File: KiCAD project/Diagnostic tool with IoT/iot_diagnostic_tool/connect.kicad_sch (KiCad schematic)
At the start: 0 parts

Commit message: Update 03/03/23 - new schematic done
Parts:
- added J5: Debug, symbol Connector_Generic:Conn_02x05_Odd_Even
- added J7: OBD, symbol Connector:Conn_01x08_Socket
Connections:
- new net +12V: J7.8 (Pin_8)
- new net +3V3: J5.1 (Pin_1)
- new net CAN_H: J7.3 (Pin_3)
- new net CAN_L: J7.4 (Pin_4)
- new net DBG_RX: J5.5 (Pin_5)
- new net DBG_TX: J5.3 (Pin_3)
- new net GND: J5.10 (Pin_10), J5.7 (Pin_7), J5.9 (Pin_9), J7.2 (Pin_2), J7.5 (Pin_5)
- new net ISO_K: J7.6 (Pin_6)
- new net ISO_L: J7.7 (Pin_7)
- new net NRST: J5.8 (Pin_8)
- new net SWCLK: J5.4 (Pin_4)
- new net SWDIO: J5.2 (Pin_2)
- new net SWO: J5.6 (Pin_6)
- no-connect marks 0 -> 1
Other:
- note added: "Connectors"
- note added: "Debug"
- note added: "OBD"

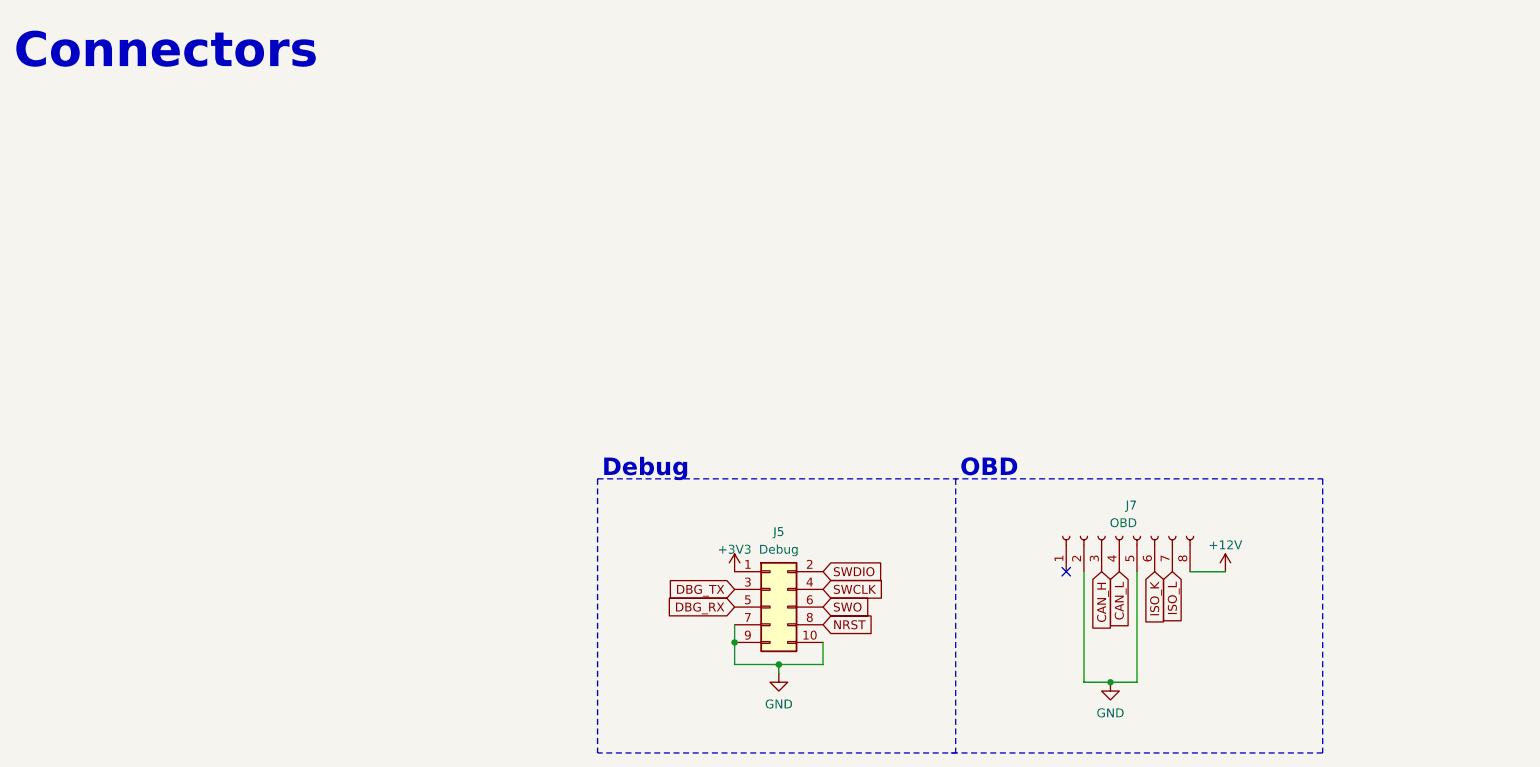
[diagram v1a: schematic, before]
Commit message: Update 06/03/23 - new board layout WIP 70%
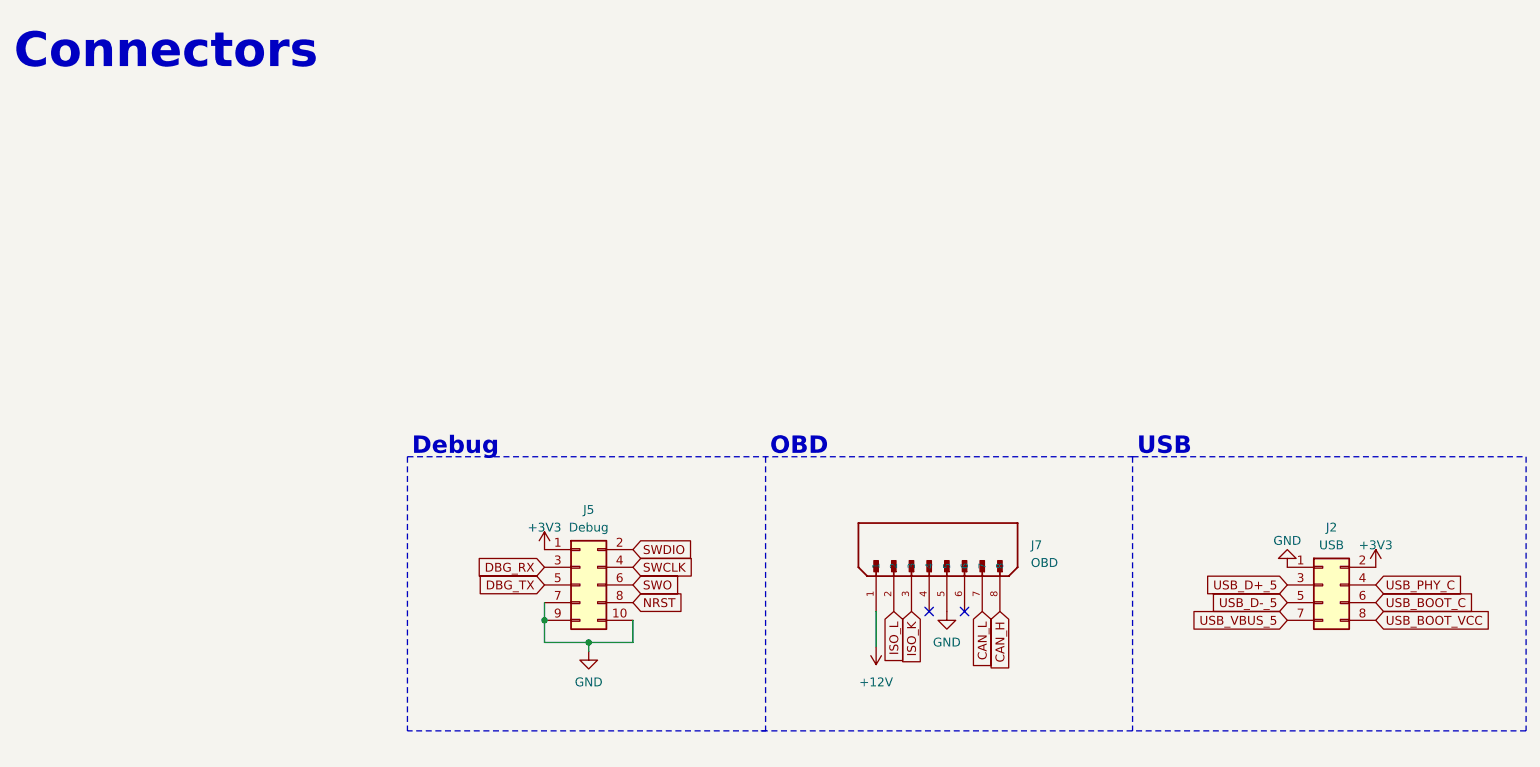
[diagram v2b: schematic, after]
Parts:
- removed J7: OBD, symbol Connector:Conn_01x08_Socket
- added J2: USB, Connector_PinHeader_2.54mm:PinHeader_2x04_P2.54mm_Vertical_SMD, symbol Connector_Generic:Conn_02x04_Odd_Even
- added J7: OBD, MOLEX_436500827, symbol 436500827:436500827
- J5: footprint (none) -> Connector_PinHeader_2.54mm:PinHeader_2x05_P2.54mm_Vertical
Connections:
- net +12V: now also J7.1
- net +3V3: now also J2.2 (Pin_2)
- net CAN_H: now also J7.8
- net CAN_L: now also J7.7
- net DBG_RX: now also J5.3 (Pin_3); no longer J5.5 (Pin_5)
- net DBG_TX: now also J5.5 (Pin_5); no longer J5.3 (Pin_3)
- net GND: now also J2.1 (Pin_1), J7.5
- net ISO_K: now also J7.3
- net ISO_L: now also J7.2
- new net USB_BOOT_C: J2.6 (Pin_6)
- new net USB_BOOT_VCC: J2.8 (Pin_8)
- new net USB_D+_5: J2.3 (Pin_3)
- new net USB_D-_5: J2.5 (Pin_5)
- new net USB_PHY_C: J2.4 (Pin_4)
- new net USB_VBUS_5: J2.7 (Pin_7)
- no-connect marks 1 -> 2
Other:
- note added: "USB"
- moved on the sheet: J5

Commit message: Update 17/03/23 - final board update, generated files for manufacturing
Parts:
- J7: footprint MOLEX_436500827 -> 436500827:MOLEX_436500827
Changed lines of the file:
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@@
       (effects (font (size 1.27 1.27)) (justify right))
     )
-    (property "Footprint" "MOLEX_436500827" (at 143.51 92.075 0)
+    (property "Footprint" "436500827:MOLEX_436500827" (at 143.51 92.075 0)
       (effects (font (size 1.27 1.27)) (justify bottom) hide)
     )

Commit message: Update 26/06/23 - Thesis release
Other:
- company: VUT -> FEKT VUT
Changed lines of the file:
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@@
     (title "OBD Monitoring Device")
     (date "2023-02-27")
-    (company "VUT")
+    (company "FEKT VUT")
   )
   (junction (at 88.265 98.425) (diameter 0) (color 0 0 0 0)
